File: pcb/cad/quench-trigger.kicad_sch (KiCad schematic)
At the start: 37 parts, among them J701 Conn_Coaxial, J702 DB9_Female, K701 FINDER-30.22, Q701 BC846B, SW701 RST, SW702 TRIG, U701 74HCS08, U702 74HC574, U703 74LV132, U704 74LVC2G17, U705 74LVC2G17, U706 HFBR-1521Z

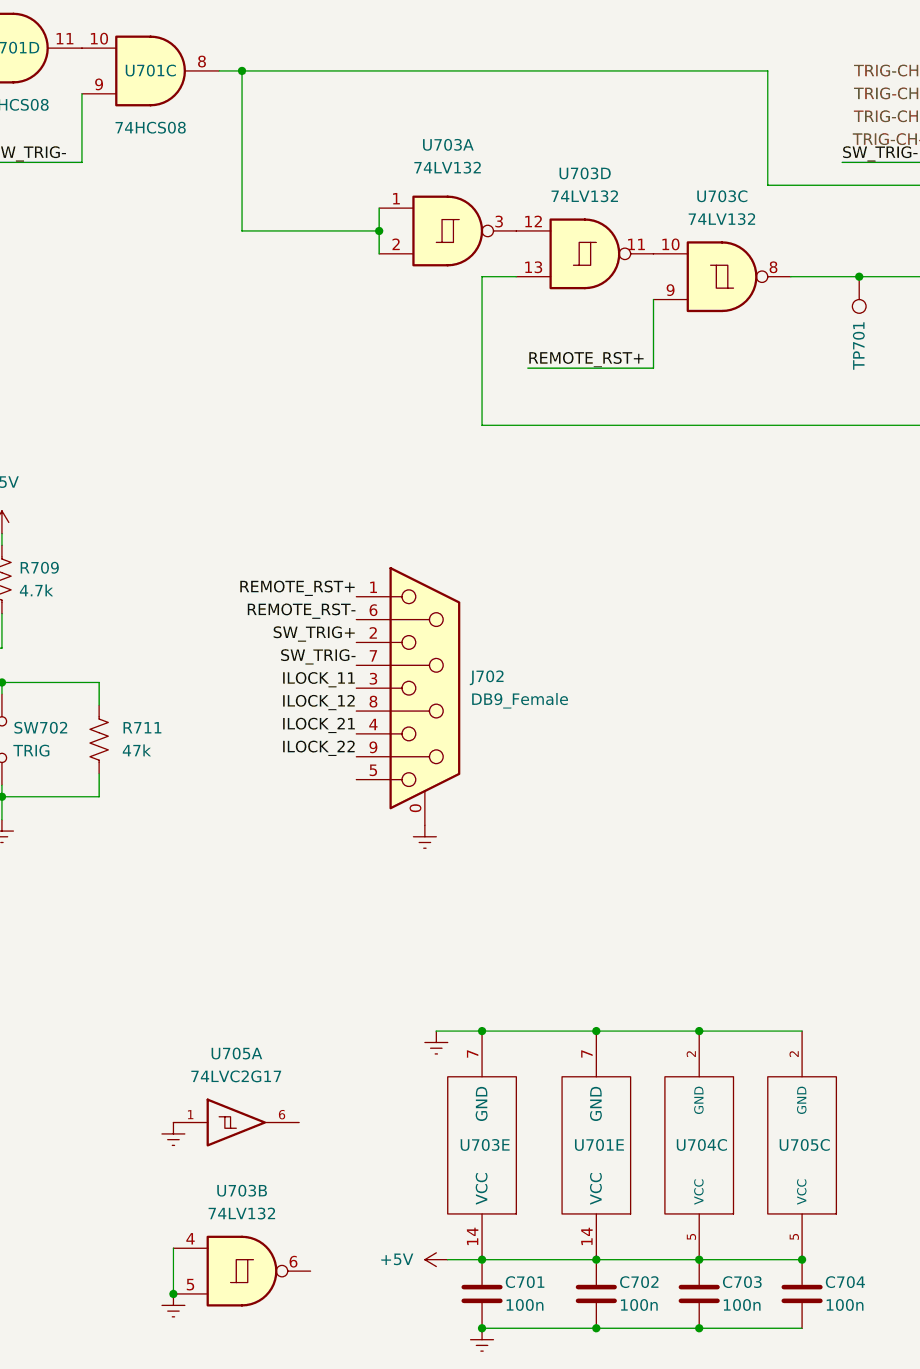
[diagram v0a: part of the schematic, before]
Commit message: Remake some logic connections and update PCB
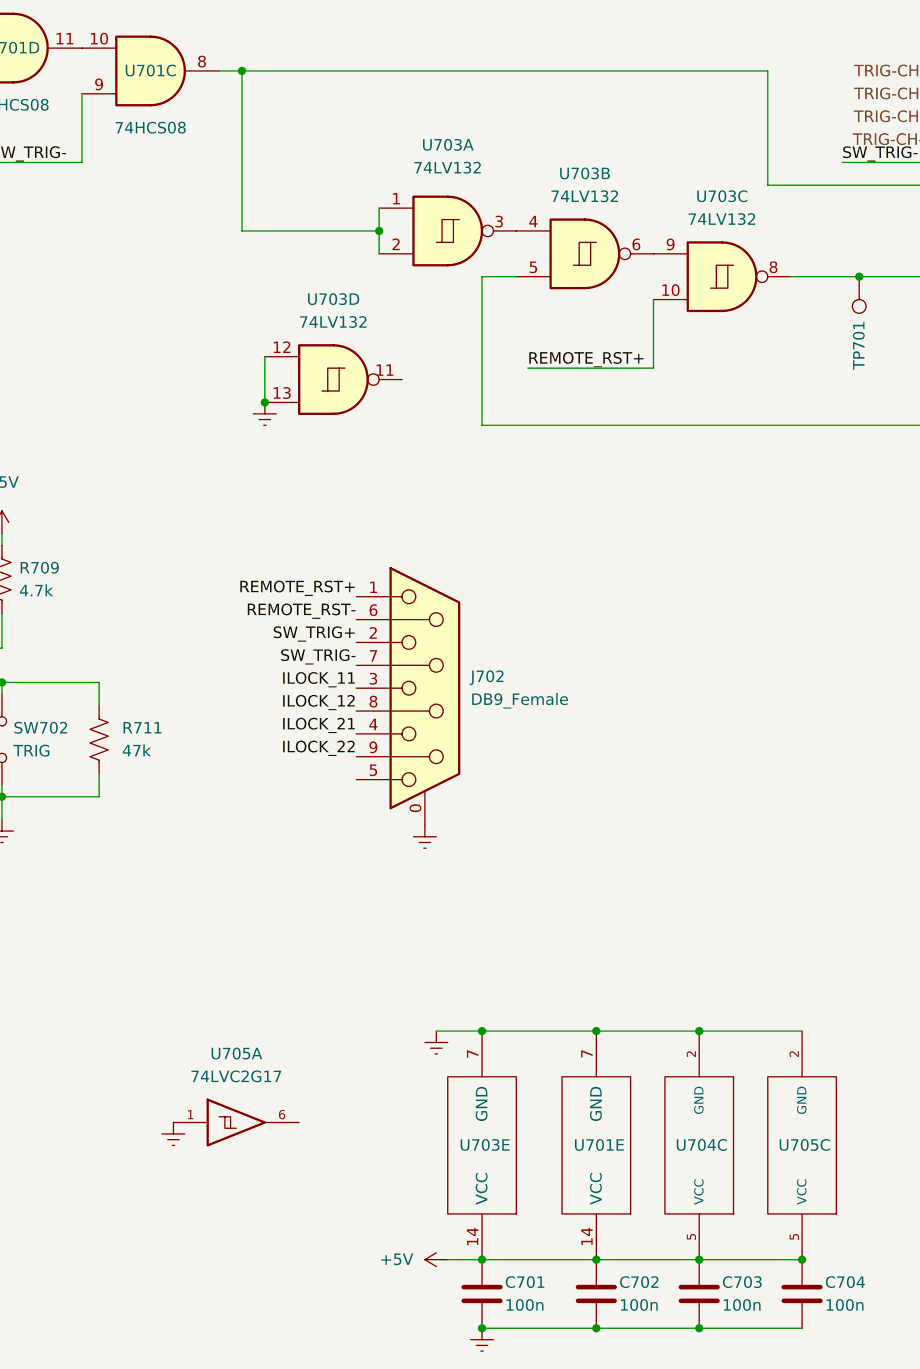
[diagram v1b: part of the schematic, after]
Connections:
- net Earth: now also U703.12, U703.13; no longer U703.4, U703.5
- net REMOTE_RST+: now also U703.10; no longer U703.9
- net at TP702.1, U702.14 (Q5), U704.1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: now also U703.5; no longer U703.13
- net at U703.3: now also U703.4; no longer U703.12
- net at U703.11: no longer U703.10
- net at U703.6: now also U703.9
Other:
- moved on the sheet: U703B, U703D
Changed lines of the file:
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@@
   (junction (at 236.22 34.925) (diameter 0) (color 0 0 0 0)
   )
-  (junction (at 87.63 187.96) (diameter 0) (color 0 0 0 0)
-  )
   (junction (at 146.05 158.75) (diameter 0) (color 0 0 0 0)
   )
@@
   (junction (at 231.14 101.6) (diameter 0) (color 0 0 0 0)
   )
+  (junction (at 97.79 88.9) (diameter 0) (color 0 0 0 0)
+  )
   (junction (at 43.815 116.205) (diameter 0) (color 0 0 0 0)
   )
@@
     (stroke (width 0) (type default) (color 0 0 0 0))
   )
-  (wire (pts (xy 87.63 182.88) (xy 87.63 187.96))
+  (wire (pts (xy 97.79 83.82) (xy 97.79 88.9))
     (stroke (width 0) (type default) (color 0 0 0 0))
   )
@@
     (pin "2")
   )
-  (symbol (lib_id "power:Earth") (at 87.63 187.96 0) (unit 1)
-    (in_bom yes) (on_board yes) (fields_autoplaced)
-    (property "Reference" "#PWR0717" (id 0) (at 87.63 194.31 0)
-      (effects (font (size 1.27 1.27)) hide)
-    )
-    (property "Value" "Earth" (id 1) (at 87.63 191.77 0)
-      (effects (font (size 1.27 1.27)) hide)
-    )
-    (property "Footprint" "" (id 2) (at 87.63 187.96 0)
-      (effects (font (size 1.27 1.27)) hide)
-    )
-    (property "Datasheet" "~" (id 3) (at 87.63 187.96 0)
+  (symbol (lib_id "power:Earth") (at 97.79 88.9 0) (unit 1)
+    (in_bom yes) (on_board yes) (fields_autoplaced)
+    (property "Reference" "#PWR0717" (id 0) (at 97.79 95.25 0)
+      (effects (font (size 1.27 1.27)) hide)
+    )
+    (property "Value" "Earth" (id 1) (at 97.79 92.71 0)
+      (effects (font (size 1.27 1.27)) hide)
+    )
+    (property "Footprint" "" (id 2) (at 97.79 88.9 0)
+      (effects (font (size 1.27 1.27)) hide)
+    )
+    (property "Datasheet" "~" (id 3) (at 97.79 88.9 0)
       (effects (font (size 1.27 1.27)) hide)
     )
@@
     (pin "7")
   )
-  (symbol (lib_name "74LV132_2") (lib_id "qds-cv-lib-sym:74LV132") (at 133.35 72.39 0) (unit 4)
-    (in_bom yes) (on_board yes) (fields_autoplaced)
-    (property "Reference" "U703" (id 0) (at 133.35 63.5 0))
-    (property "Value" "74LV132" (id 1) (at 133.35 66.04 0))
-    (property "Footprint" "Package_SO:SO-14_3.9x8.65mm_P1.27mm" (id 2) (at 133.35 72.39 0)
-      (effects (font (size 1.27 1.27)) hide)
-    )
-    (property "Datasheet" "http://www.ti.com/lit/ds/symlink/sn74lv132a.pdf" (id 3) (at 133.35 72.39 0)
-      (effects (font (size 1.27 1.27)) hide)
-    )
-    (property "Part Number" "SN74LV132ADR" (id 4) (at 133.35 72.39 0)
+  (symbol (lib_name "74LV132_2") (lib_id "qds-cv-lib-sym:74LV132") (at 105.41 86.36 0) (unit 4)
+    (in_bom yes) (on_board yes) (fields_autoplaced)
+    (property "Reference" "U703" (id 0) (at 105.41 77.47 0))
+    (property "Value" "74LV132" (id 1) (at 105.41 80.01 0))
+    (property "Footprint" "Package_SO:SO-14_3.9x8.65mm_P1.27mm" (id 2) (at 105.41 86.36 0)
+      (effects (font (size 1.27 1.27)) hide)
+    )
+    (property "Datasheet" "http://www.ti.com/lit/ds/symlink/sn74lv132a.pdf" (id 3) (at 105.41 86.36 0)
+      (effects (font (size 1.27 1.27)) hide)
+    )
+    (property "Part Number" "SN74LV132ADR" (id 4) (at 105.41 86.36 0)
       (effects (font (size 1.27 1.27)) hide)
     )
@@
     (pin "1")
   )
-  (symbol (lib_name "74LV132_4") (lib_id "qds-cv-lib-sym:74LV132") (at 148.59 74.93 0) (mirror x) (unit 3)
+  (symbol (lib_name "74LV132_4") (lib_id "qds-cv-lib-sym:74LV132") (at 148.59 74.93 0) (unit 3)
     (in_bom yes) (on_board yes) (fields_autoplaced)
     (property "Reference" "U703" (id 0) (at 148.59 66.04 0))
@@
     (pin "3")
   )
-  (symbol (lib_id "qds-cv-lib-sym:74LV132") (at 95.25 185.42 0) (unit 2)
-    (in_bom yes) (on_board yes) (fields_autoplaced)
-    (property "Reference" "U703" (id 0) (at 95.25 176.53 0))
-    (property "Value" "74LV132" (id 1) (at 95.25 179.07 0))
-    (property "Footprint" "Package_SO:SO-14_3.9x8.65mm_P1.27mm" (id 2) (at 95.25 185.42 0)
-      (effects (font (size 1.27 1.27)) hide)
-    )
-    (property "Datasheet" "http://www.ti.com/lit/ds/symlink/sn74lv132a.pdf" (id 3) (at 95.25 185.42 0)
-      (effects (font (size 1.27 1.27)) hide)
-    )
-    (property "Part Number" "SN74LV132ADR" (id 4) (at 95.25 185.42 0)
-      (effects (font (size 1.27 1.27)) hide)
-    )
+  (symbol (lib_id "qds-cv-lib-sym:74LV132") (at 133.35 72.39 0) (unit 2)
+    (in_bom yes) (on_board yes) (fields_autoplaced)
+    (property "Reference" "U703" (id 0) (at 133.35 63.5 0))
+    (property "Value" "74LV132" (id 1) (at 133.35 66.04 0))
+    (property "Footprint" "Package_SO:SO-14_3.9x8.65mm_P1.27mm" (id 2) (at 133.35 72.39 0)
+      (effects (font (size 1.27 1.27)) hide)
+    )
+    (property "Datasheet" "http://www.ti.com/lit/ds/symlink/sn74lv132a.pdf" (id 3) (at 133.35 72.39 0)
+      (effects (font (size 1.27 1.27)) hide)
+    )
+    (property "Part Number" "SN74LV132ADR" (id 4) (at 133.35 72.39 0)
+      (effects (font (size 1.27 1.27)) hide)
+    )
